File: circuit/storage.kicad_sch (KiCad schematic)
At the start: 15 parts, among them J1 Port B, J2 Port C, J25 SPI programmer, J3 SDCard, J4 Port A, J43 Port G, U10 74HC74, U3 4081

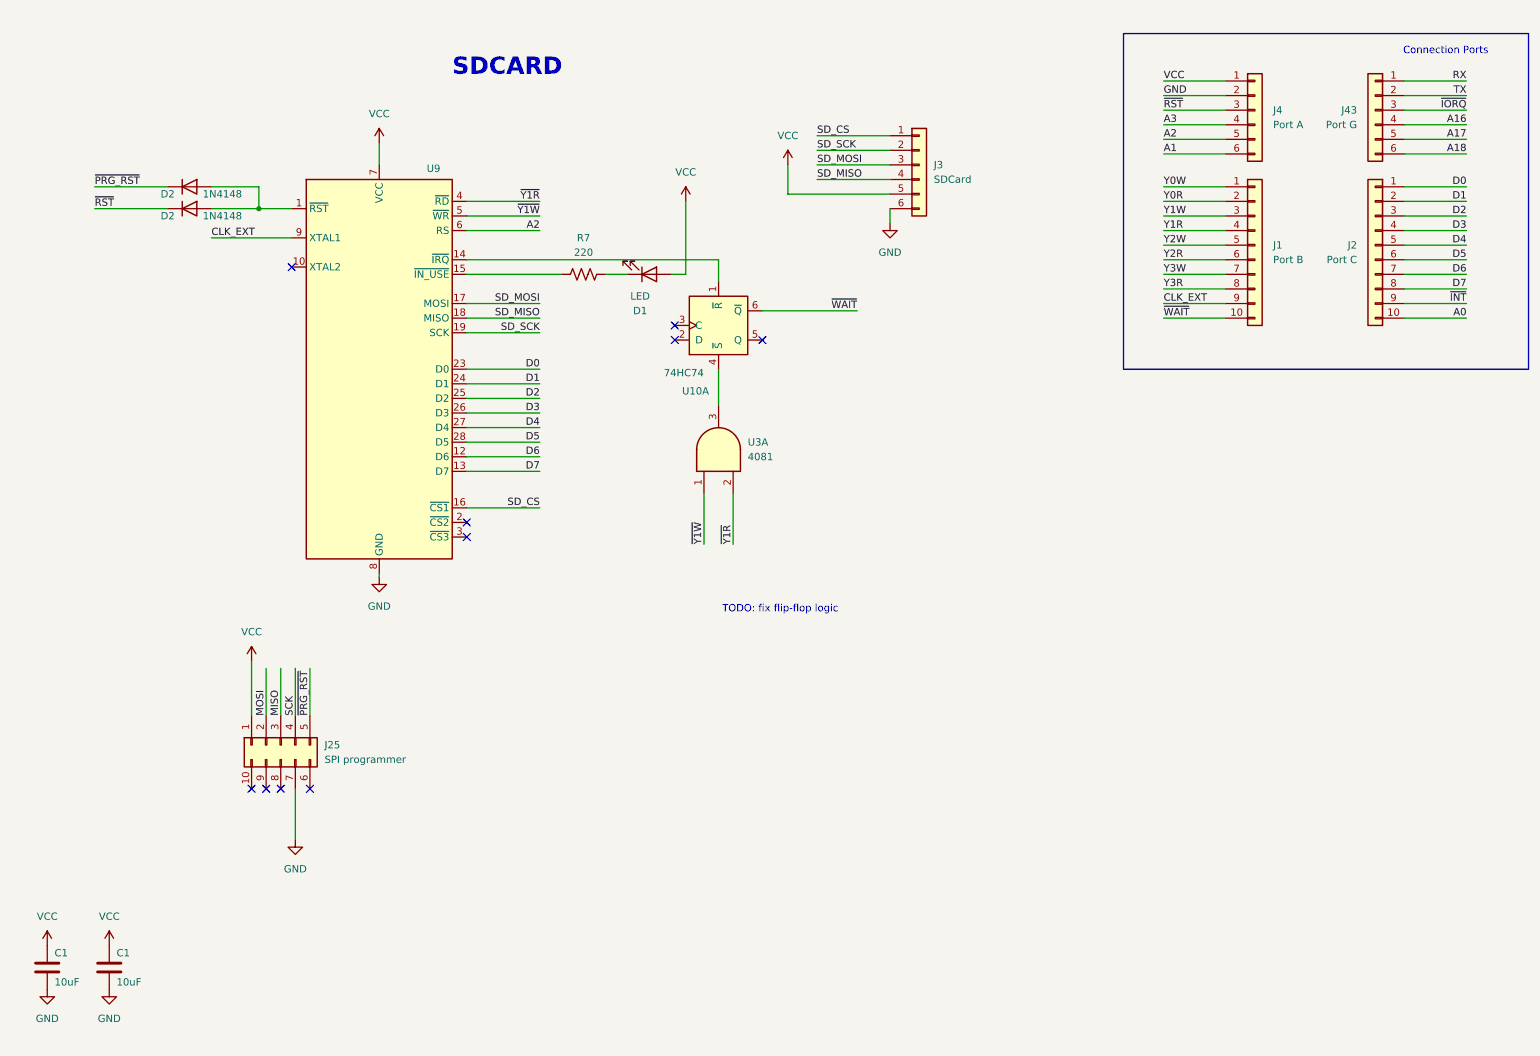
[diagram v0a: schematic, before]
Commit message: .
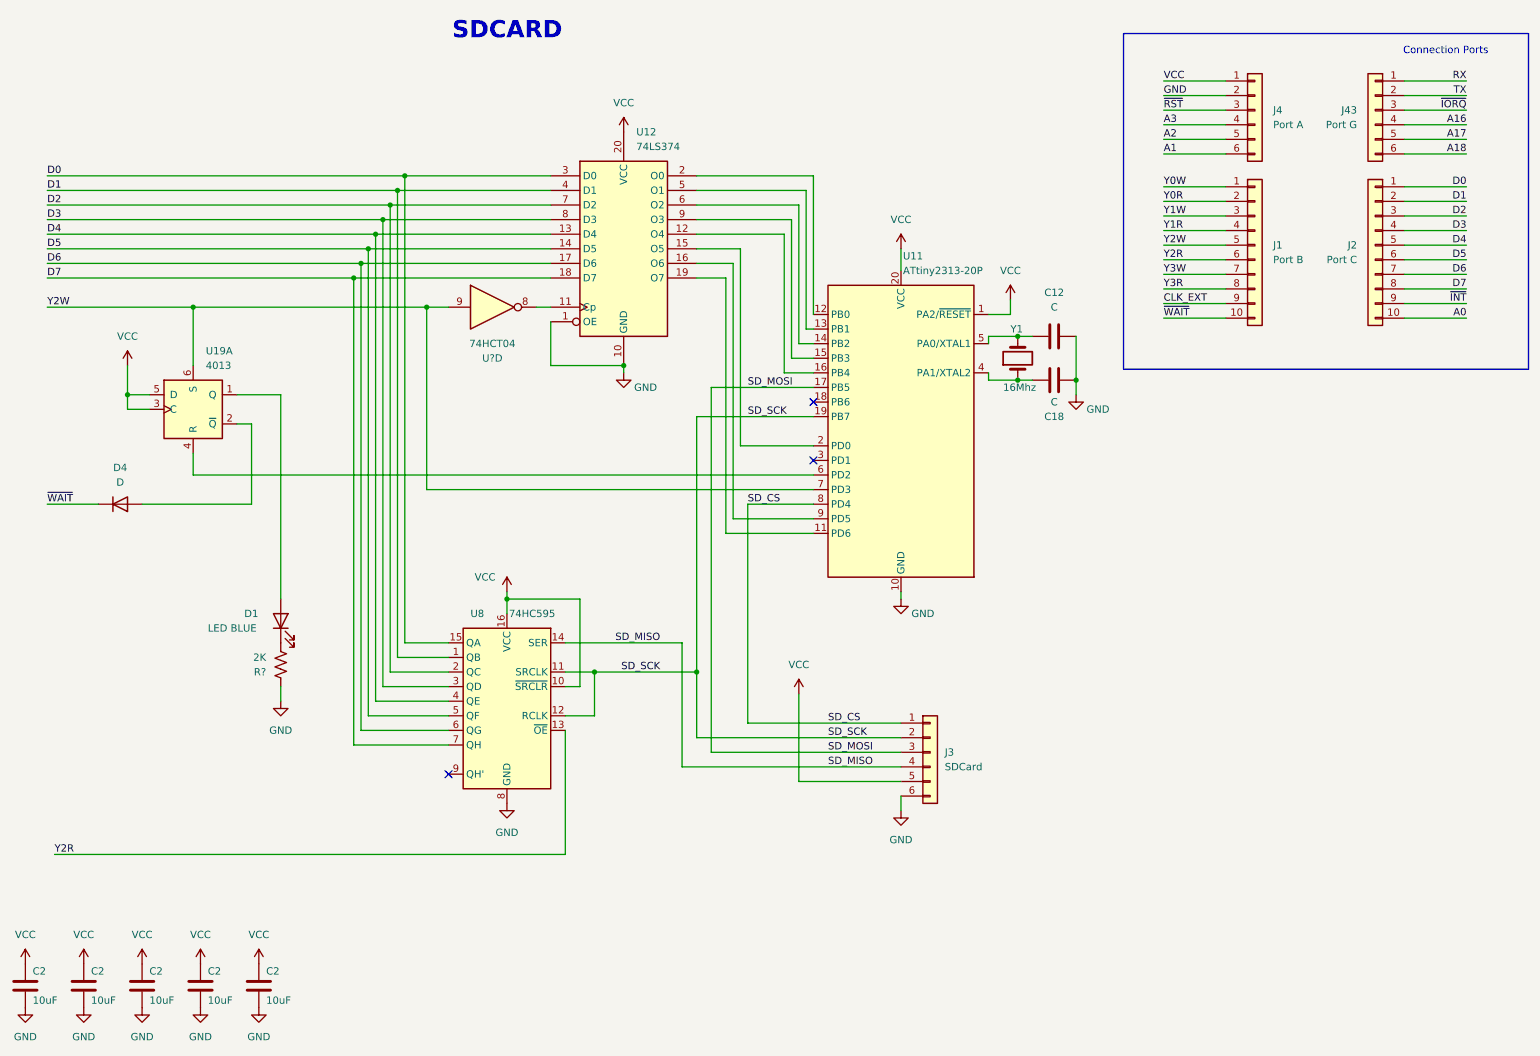
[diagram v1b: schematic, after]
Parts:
- removed C1 (x2): 10uF, symbol Device:C
- removed D2 (x2): 1N4148, Diode_THT:D_DO-35_SOD27_P7.62mm_Horizontal, symbol Diode:1N4148
- removed J25: SPI programmer, symbol Connector_Generic:Conn_02x05_Counter_Clockwise
- removed R7: 220, symbol Device:R_US
- removed U10: 74HC74, symbol 74xx:74HC74
- removed U3: 4081, symbol 4xxx:4081
- removed U9: ~, symbol parallel-to-spi:Parallel_to_SPI
- added C12, C18: C, symbol Device:C
- added C2 (x5): 10uF, symbol Device:C
- added D4: D, symbol Device:D
- added R?: 2K, symbol Device:R_US
- added U11: ATtiny2313-20P, Package_DIP:DIP-20_W7.62mm, symbol MCU_Microchip_ATtiny:ATtiny2313-20P
- added U12: 74LS374, symbol 74xx:74LS374
- added U19: 4013, symbol 4xxx:4013
- added U8: 74HC595, symbol 74xx:74HC595
- added U?: 74HCT04, symbol 74xx:74HCT04
- added Y1: 16Mhz, symbol Device:Crystal
- D1: value LED -> LED BLUE
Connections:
- net D0: now also U12.3 (D0), U8.15 (QA)
- net D1: now also U12.4 (D1), U8.1 (QB)
- net D2: now also U12.7 (D2), U8.2 (QC)
- net D3: now also U12.8 (D3), U8.3 (QD)
- net D4: now also U12.13 (D4), U8.4 (QE)
- net D5: now also U12.14 (D5), U8.5 (QF)
- net D6: now also U12.17 (D6), U8.6 (QG)
- net D7: now also U12.18 (D7), U8.7 (QH)
- net GND: now also C12.2, C18.2, C2.2, C2.2, C2.2, C2.2, C2.2, R?.2, U11.10 (GND), U12.1 (OE), U12.10 (GND), U8.8 (GND)
- net SD_CS: now also U11.8 (PD4)
- net SD_MISO: now also U8.14 (SER)
- net SD_MOSI: now also U11.17 (PB5)
- net SD_SCK: now also U11.19 (PB7), U8.11 (SRCLK), U8.12 (RCLK)
- net VCC: now also C2.1, C2.1, C2.1, C2.1, C2.1, U11.1 (PA2/~{RESET}), U11.20 (VCC), U12.20 (VCC), U19.3 (C), U19.5 (D), U8.10 (~{SRCLR}), U8.16 (VCC); no longer D1.2 (A)
- net Y2R: now also U8.13 (~{OE})
- net Y2W: now also U11.7 (PD3), U19.6 (S), U?.9
- net ~{WAIT}: now also D4.1 (K)
- net at D1.1 (K): now also R?.1
- new net: C12.1, U11.5 (PA0/XTAL1), Y1.2
- new net: U12.11 (Cp), U?.8
- new net: U11.16 (PB4), U12.12 (O4)
- new net: U11.2 (PD0), U12.15 (O5)
- new net: U11.9 (PD5), U12.16 (O6)
- new net: U11.11 (PD6), U12.19 (O7)
- new net: U11.12 (PB0), U12.2 (O0)
- new net: U11.13 (PB1), U12.5 (O1)
- new net: U11.14 (PB2), U12.6 (O2)
- new net: U11.15 (PB3), U12.9 (O3)
- new net: D1.2 (A), U19.1 (Q)
- new net: C18.1, U11.4 (PA1/XTAL2), Y1.1
- new net: U11.6 (PD2), U19.4 (R)
- new net: D4.2 (A), U19.2 (~{Q})
- no-connect marks 10 -> 3
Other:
- note removed: "TODO: fix flip-flop logic"
- moved on the sheet: J3
